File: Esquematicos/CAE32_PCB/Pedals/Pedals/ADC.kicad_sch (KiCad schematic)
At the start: 16 parts, among them J10 Conn_01x03_Female, J11 Conn_01x03_Female, J12 Conn_01x03_Female, J13 Conn_01x03_Female, J14 Conn_01x03_Female, J4 Conn_01x03_Female, J5 Conn_01x03_Female, J6 Conn_01x03_Female, J7 Conn_01x03_Female, J8 Conn_01x03_Female, J9 Conn_01x03_Female, U2 REF3033, U3 ADC128S102

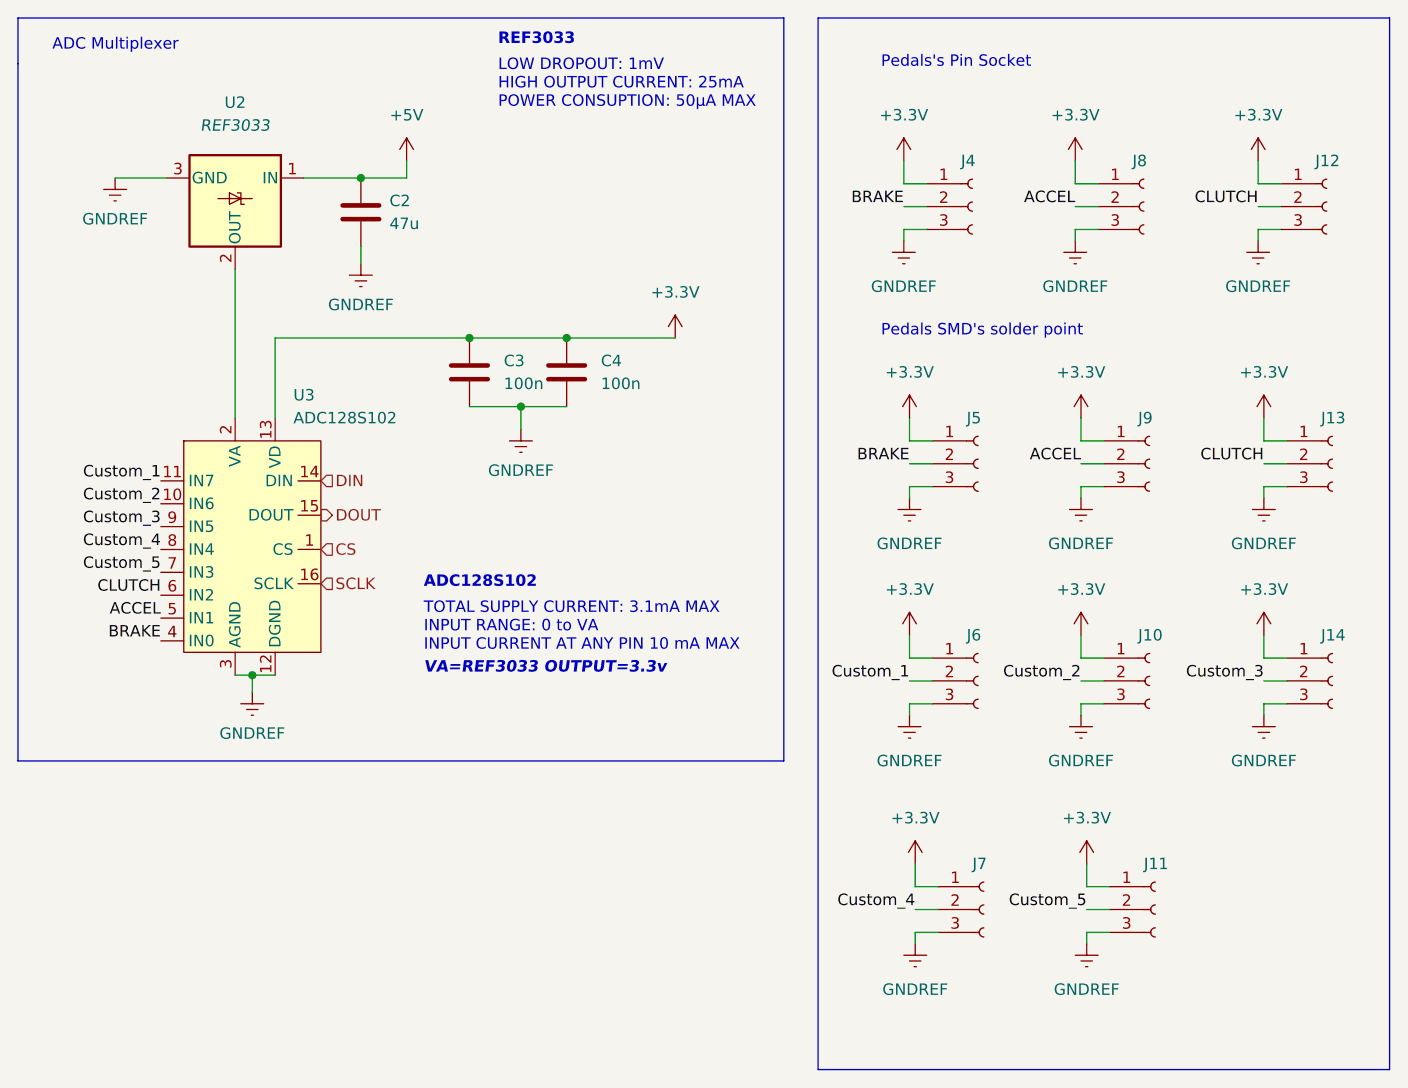
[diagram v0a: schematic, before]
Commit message: chore: arrange schematics components
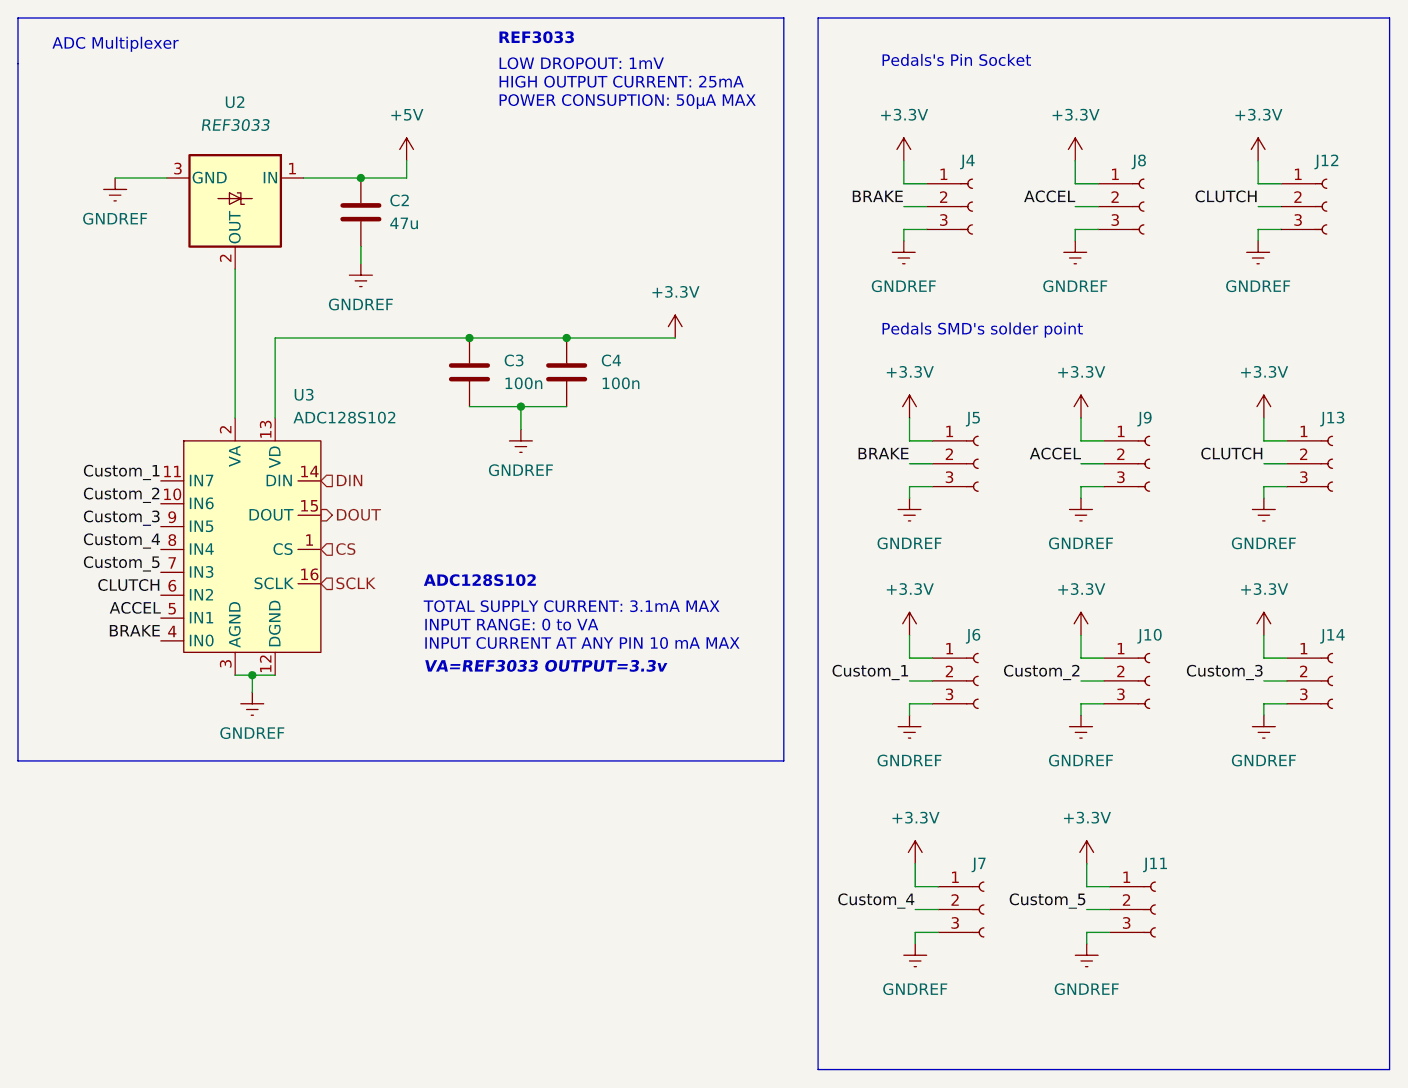
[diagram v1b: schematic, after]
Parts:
- C2, C3, C4: footprint Capacitor_SMD:C_0603_1608Metric_Pad1.08x0.95mm_HandSolder -> Capacitor_SMD:C_0603_1608Metric
